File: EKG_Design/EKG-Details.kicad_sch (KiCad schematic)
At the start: 14 parts

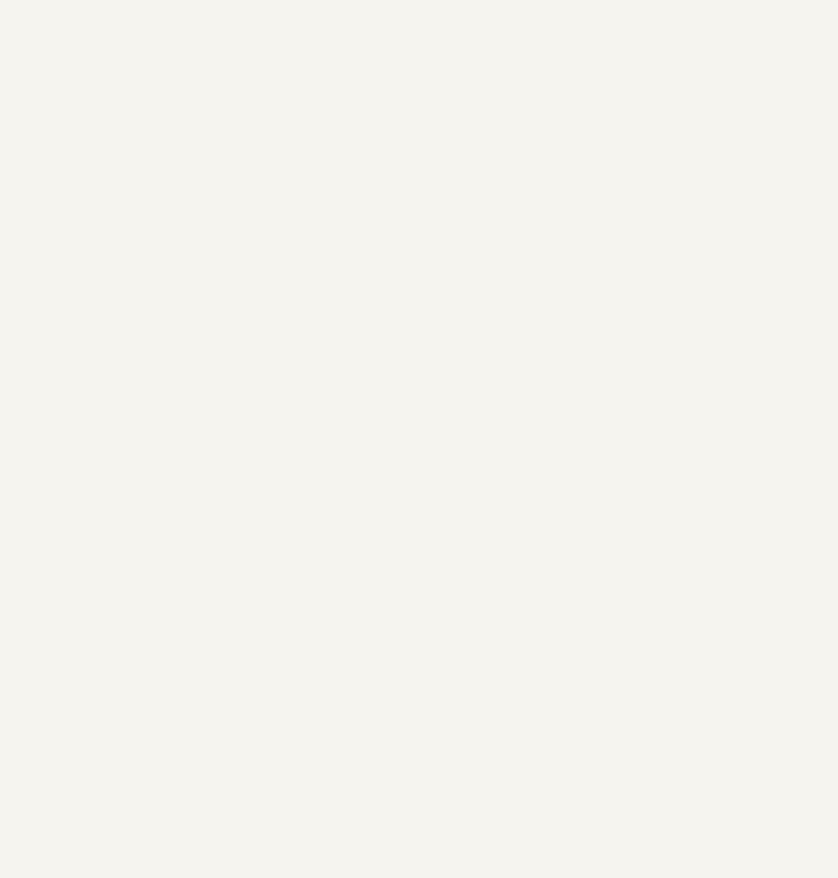
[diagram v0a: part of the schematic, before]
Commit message: EKG-Details updated
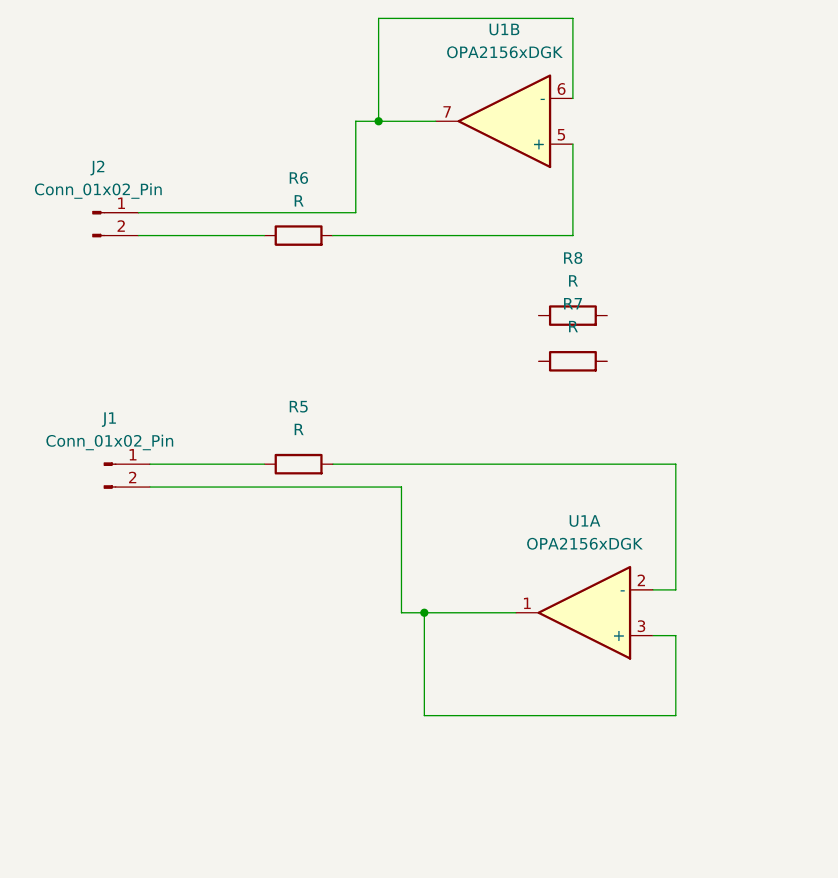
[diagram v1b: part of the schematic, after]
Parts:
- added J1, J2: Conn_01x02_Pin, symbol Connector:Conn_01x02_Pin
- added R5, R6, R7, R8: R, symbol Device:R
- added U1: OPA2156xDGK, Package_SO:VSSOP-8_3x3mm_P0.65mm, symbol Amplifier_Operational:OPA2156xDGK
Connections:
- new net: R6.2, U1.5 (+)
- new net: J2.1 (Pin_1), U1.6 (-), U1.7
- new net: J1.1 (Pin_1), R5.1
- new net: R5.2, U1.2 (-)
- new net: J1.2 (Pin_2), U1.1, U1.3 (+)
- new net: J2.2 (Pin_2), R6.1
